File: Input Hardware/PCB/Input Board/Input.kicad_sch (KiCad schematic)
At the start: 28 parts, among them SW1501 Rotary encoder, SW1502 Rotary encoder, U1501 74HC595

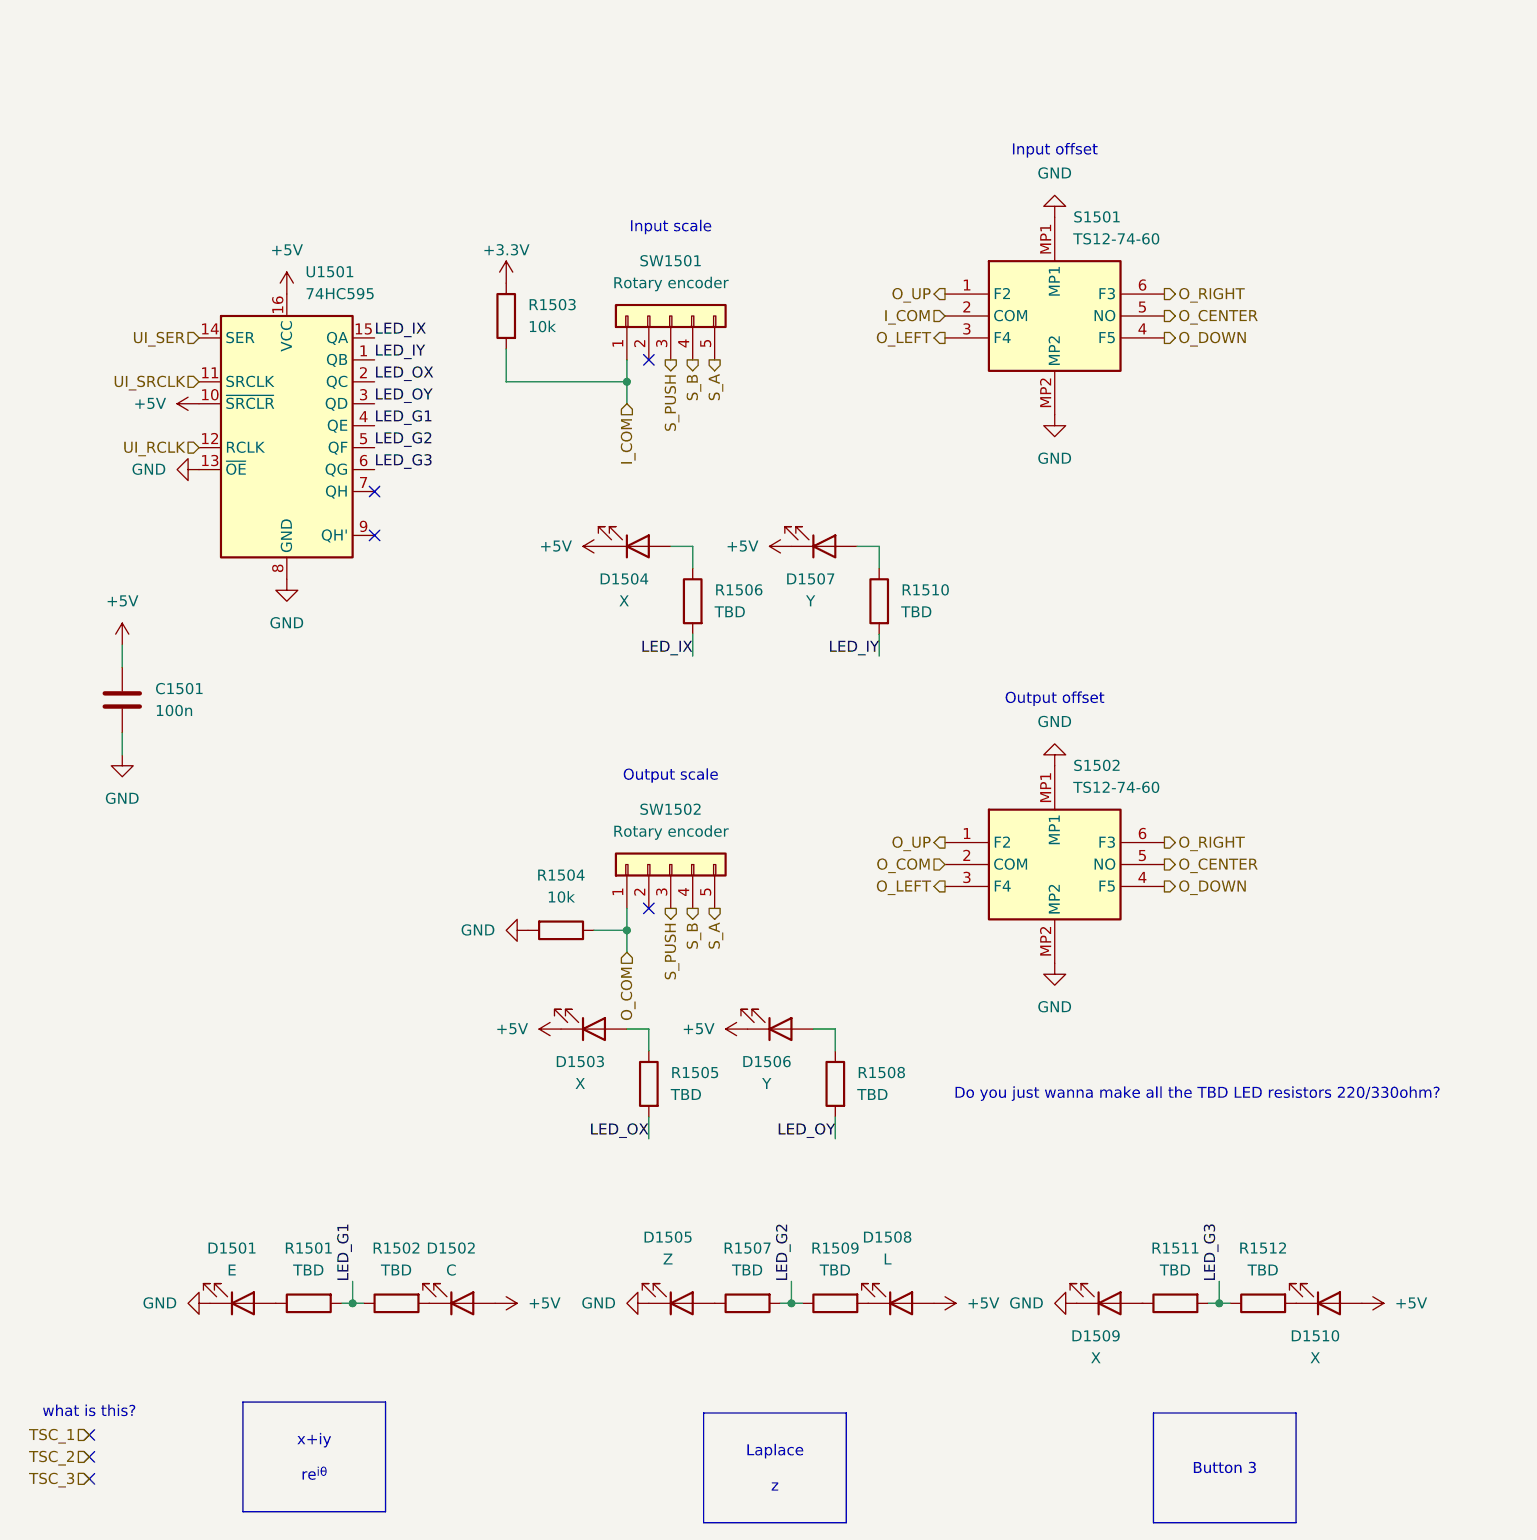
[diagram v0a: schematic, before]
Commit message: minor schematic changes and value assignment
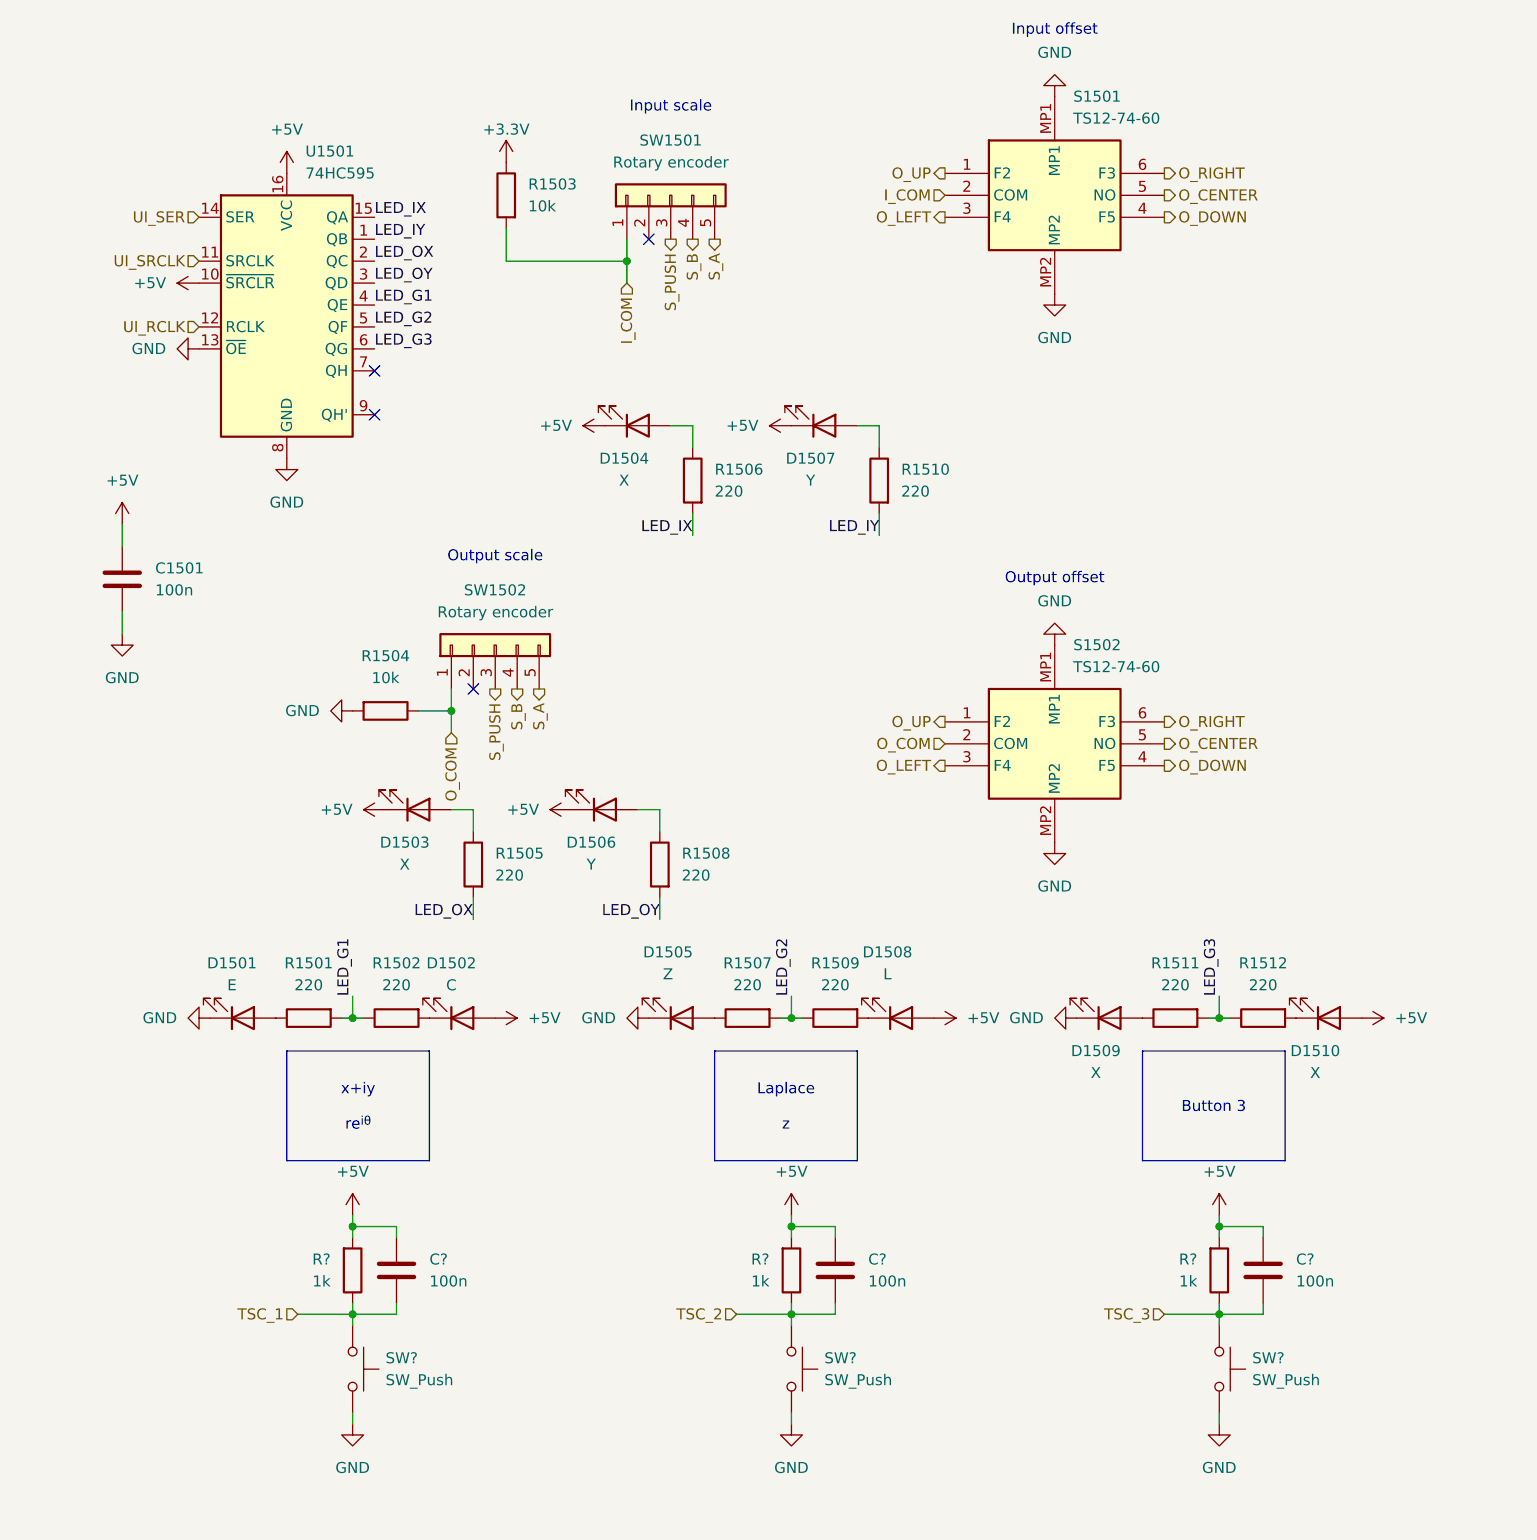
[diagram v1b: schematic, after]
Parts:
- added C? (x3): 100n, Capacitor_SMD:C_0603_1608Metric, symbol Device:C
- added R? (x3): 1k, Resistor_SMD:R_0603_1608Metric, symbol Device:R
- added SW? (x3): SW_Push, Button_Switch_SMD:SW_SPST_B3S-1000, symbol Switch:SW_Push
- R1501, R1502, R1505, R1506, R1507, R1508, R1509, R1510, R1511, R1512: value TBD -> 220
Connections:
- net +5V: now also C?.1, C?.1, C?.1, R?.2, R?.2, R?.2
- net GND: now also SW?.2, SW?.2, SW?.2
- net TSC_1: now also C?.2, R?.1, SW?.1
- net TSC_2: now also C?.2, R?.1, SW?.1
- net TSC_3: now also C?.2, R?.1, SW?.1
- no-connect marks 7 -> 4
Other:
- note removed: "Do you just wanna make all the TBD LED resistors 220/330ohm?"
- note removed: "what is this?"
- moved on the sheet: C1501, D1501, D1502, D1503, D1504, D1505, D1506, D1507, D1508, D1509, D1510, R1501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
